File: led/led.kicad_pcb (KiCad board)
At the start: 2 copper layers, 11 x 9 mm, 3 parts

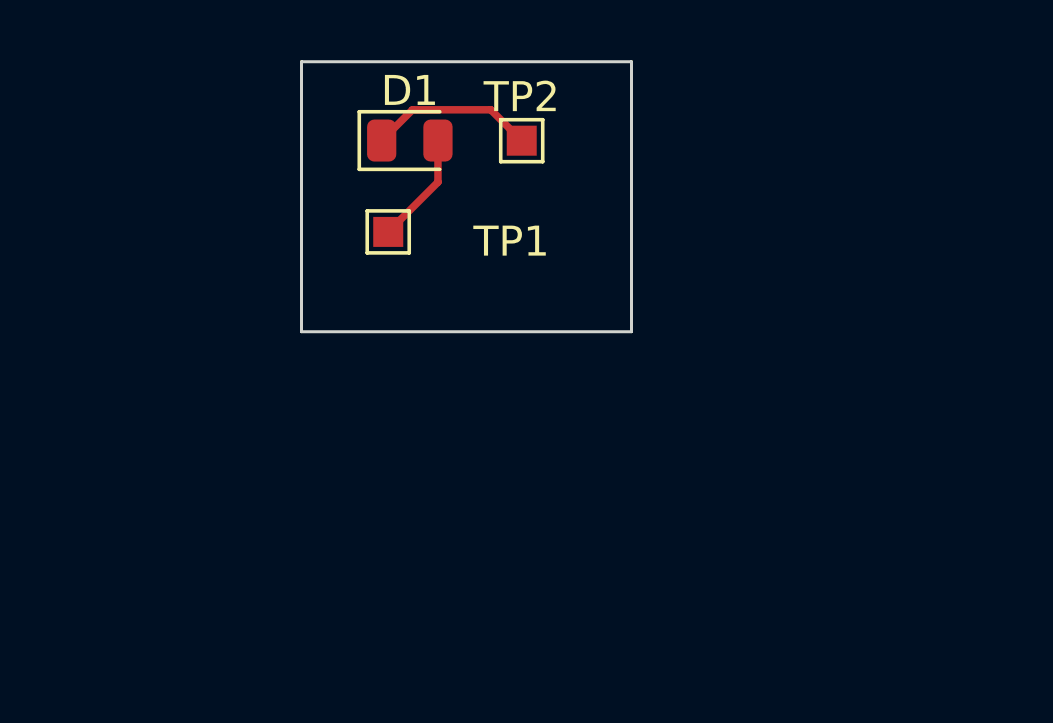
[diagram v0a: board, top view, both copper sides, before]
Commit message: led
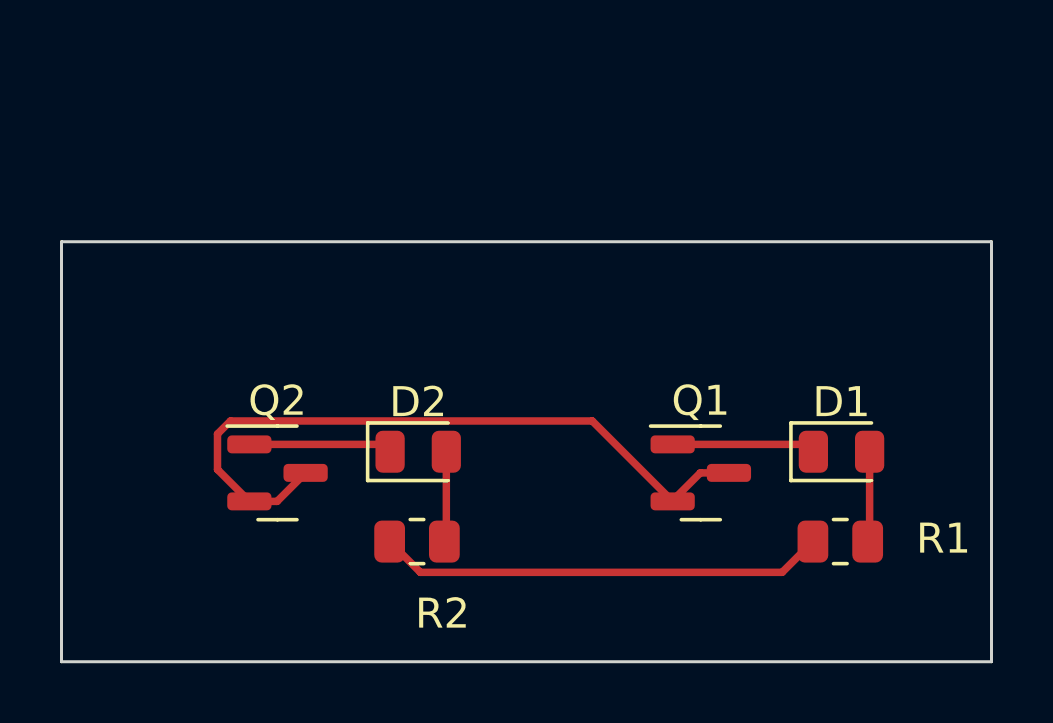
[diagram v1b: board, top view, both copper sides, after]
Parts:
- removed TP1, TP2: TestPoint, TestPoint:TestPoint_Pad_1.0x1.0mm
- added D2: LED, LED_SMD:LED_0805_2012Metric, F.Cu at (162.9, 101.0)
- added Q1: Q_NMOS_DGS, Package_TO_SOT_SMD:SOT-23, F.Cu at (172.3, 101.7)
- added Q2: Q_NMOS_DGS, Package_TO_SOT_SMD:SOT-23, F.Cu at (158.2, 101.7)
- added R1: R, Resistor_SMD:R_0805_2012Metric, F.Cu at (177.0, 104.0)
- added R2: R, Resistor_SMD:R_0805_2012Metric, F.Cu at (162.8, 104.0)
- moved D1 17.7 mm to (177.0, 101.0)
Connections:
- D1 pad 1: /LED_C -> /led/switched
- D1 pad 2: /LED_A -> Net-(D1-Pad2)
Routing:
- net GND: track 0.00 -> 23.7 mm
- net +3V3: track 0.00 -> 15.0 mm
- net /LED_C: track 5.52 -> 0.00 mm
- net /led1/switched: track 0.00 -> 4.79 mm
- net /led/switched: track 0.00 -> 4.79 mm
- net /LED_A: track 3.73 -> 0.00 mm
- net Net-(D2-Pad2): track 0.00 -> 3.02 mm
- net Net-(D1-Pad2): track 0.00 -> 3.02 mm
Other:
- board size 11 x 9 mm -> 31 x 14 mm
